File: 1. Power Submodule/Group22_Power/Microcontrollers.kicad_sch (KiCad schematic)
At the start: 3 parts, among them J4 Conn_01x08_Male, J5 Conn_01x08_Male, J7 GPIO

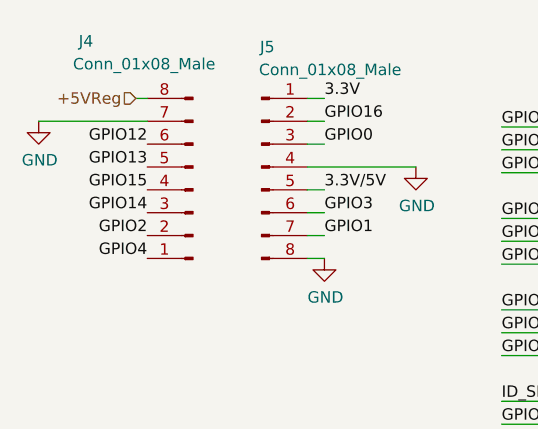
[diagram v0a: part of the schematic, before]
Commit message: $1
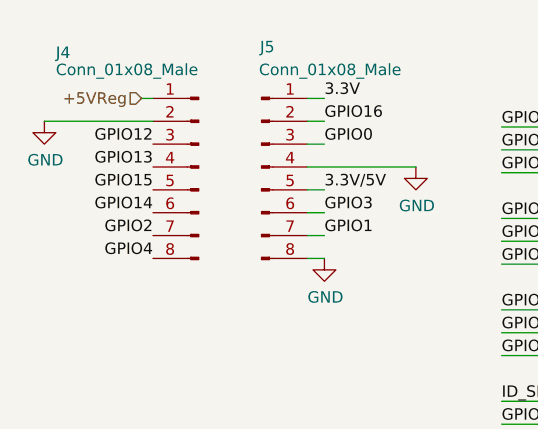
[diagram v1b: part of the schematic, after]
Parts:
- J4, J5: footprint Connector_PinHeader_2.54mm:PinHeader_1x08_P2.54mm_Vertical -> Connector_PinSocket_2.54mm:PinSocket_1x08_P2.54mm_Vertical
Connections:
- net +5VReg: now also J4.1 (Pin_1); no longer J4.8 (Pin_8)
- net GND: now also J4.2 (Pin_2); no longer J4.7 (Pin_7)
- net GPIO12: now also J4.3 (Pin_3); no longer J4.6 (Pin_6)
- net GPIO13: now also J4.4 (Pin_4); no longer J4.5 (Pin_5)
- net GPIO14: now also J4.6 (Pin_6); no longer J4.3 (Pin_3)
- net GPIO15: now also J4.5 (Pin_5); no longer J4.4 (Pin_4)
- net GPIO2: now also J4.7 (Pin_7); no longer J4.2 (Pin_2)
- net GPIO4: now also J4.8 (Pin_8); no longer J4.1 (Pin_1)
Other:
- moved on the sheet: J4
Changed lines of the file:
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@@
     (stroke (width 0) (type solid) (color 0 0 0 0))
-  )
-  (wire (pts (xy 166.37 97.79) (xy 167.64 97.79))
-    (stroke (width 0) (type default) (color 0 0 0 0))
   )
   (wire (pts (xy 248.92 144.145) (xy 275.59 144.145))
@@
     (stroke (width 0) (type default) (color 0 0 0 0))
   )
+  (wire (pts (xy 156.21 100.33) (xy 168.275 100.33))
+    (stroke (width 0) (type default) (color 0 0 0 0))
+  )
   (wire (pts (xy 251.46 90.17) (xy 251.46 98.425))
     (stroke (width 0) (type solid) (color 0 0 0 0))
@@
     (stroke (width 0) (type solid) (color 0 0 0 0))
   )
+  (wire (pts (xy 167.005 97.79) (xy 168.275 97.79))
+    (stroke (width 0) (type default) (color 0 0 0 0))
+  )
   (wire (pts (xy 236.22 121.285) (xy 207.01 121.285))
     (stroke (width 0) (type solid) (color 0 0 0 0))
@@
     (stroke (width 0) (type solid) (color 0 0 0 0))
   )
-  (wire (pts (xy 155.575 100.33) (xy 167.64 100.33))
-    (stroke (width 0) (type default) (color 0 0 0 0))
-  )
   (wire (pts (xy 231.14 98.425) (xy 236.22 98.425))
     (stroke (width 0) (type solid) (color 0 0 0 0))
@@
     (effects (font (size 1.27 1.27)) (justify left bottom))
   )
-  (label "GPIO4" (at 167.64 115.57 180)
-    (effects (font (size 1.27 1.27)) (justify right bottom))
-  )
-  (label "GPIO12" (at 167.64 102.87 180)
+  (label "GPIO13" (at 168.275 105.41 180)
     (effects (font (size 1.27 1.27)) (justify right bottom))
   )
@@
     (effects (font (size 1.27 1.27)) (justify left bottom))
   )
-  (label "GPIO13" (at 167.64 105.41 180)
-    (effects (font (size 1.27 1.27)) (justify right bottom))
-  )
   (label "GPIO0" (at 187.325 102.87 0)
     (effects (font (size 1.27 1.27)) (justify left bottom))
   )
+  (label "GPIO12" (at 168.275 102.87 180)
+    (effects (font (size 1.27 1.27)) (justify right bottom))
+  )
   (label "GPIO1" (at 187.325 113.03 0)
     (effects (font (size 1.27 1.27)) (justify left bottom))
@@
     (effects (font (size 1.27 1.27)) (justify left bottom))
   )
+  (label "GPIO2" (at 168.275 113.03 180)
+    (effects (font (size 1.27 1.27)) (justify right bottom))
+  )
   (label "GPIO[24]" (at 275.59 118.745 180)
     (effects (font (size 1.27 1.27)) (justify right bottom))
@@
     (effects (font (size 1.27 1.27)) (justify right bottom))
   )
-  (label "GPIO15" (at 167.64 107.95 180)
+  (label "GPIO14" (at 168.275 110.49 180)
     (effects (font (size 1.27 1.27)) (justify right bottom))
   )
@@
     (effects (font (size 1.27 1.27)) (justify left bottom))
   )
+  (label "GPIO4" (at 168.275 115.57 180)
+    (effects (font (size 1.27 1.27)) (justify right bottom))
+  )
   (label "GPIO[27]" (at 207.01 113.665 0)
     (effects (font (size 1.27 1.27)) (justify left bottom))
@@
     (effects (font (size 1.27 1.27)) (justify left bottom))
   )
-  (label "GPIO2" (at 167.64 113.03 180)
+  (label "GPIO15" (at 168.275 107.95 180)
     (effects (font (size 1.27 1.27)) (justify right bottom))
   )
@@
     (effects (font (size 1.27 1.27)) (justify right bottom))
   )
-  (label "GPIO14" (at 167.64 110.49 180)
-    (effects (font (size 1.27 1.27)) (justify right bottom))
-  )
   (label "GPIO[5]" (at 207.01 133.985 0)
     (effects (font (size 1.27 1.27)) (justify left bottom))
@@
     (effects (font (size 1.27 1.27)) (justify left bottom))
   )
-  (hierarchical_label "+5VReg" (shape input) (at 166.37 97.79 180)
+  (hierarchical_label "+5VReg" (shape input) (at 167.005 97.79 180)
     (effects (font (size 1.27 1.27)) (justify right))
   )
@@
     (property "Reference" "J5" (id 0) (at 180.975 92.075 0))
     (property "Value" "Conn_01x08_Male" (id 1) (at 187.96 94.615 0))
-    (property "Footprint" "Connector_PinHeader_2.54mm:PinHeader_1x08_P2.54mm_Vertical" (id 2) (at 180.34 105.41 0)
+    (property "Footprint" "Connector_PinSocket_2.54mm:PinSocket_1x08_P2.54mm_Vertical" (id 2) (at 180.34 105.41 0)
       (effects (font (size 1.27 1.27)) hide)
     )
@@
     (pin "8")
   )
-  (symbol (lib_id "Connector:Conn_01x08_Male") (at 172.72 107.95 180) (unit 1)
-    (in_bom yes) (on_board yes)
-    (property "Reference" "J4" (id 0) (at 160.02 91.44 0)
+  (symbol (lib_id "Connector:Conn_01x08_Male") (at 173.355 105.41 0) (mirror y) (unit 1)
+    (in_bom yes) (on_board yes)
+    (property "Reference" "J4" (id 0) (at 157.48 92.71 0)
       (effects (font (size 1.27 1.27)) (justify right))
     )
-    (property "Value" "Conn_01x08_Male" (id 1) (at 159.385 93.98 0)
+    (property "Value" "Conn_01x08_Male" (id 1) (at 157.48 94.615 0)
       (effects (font (size 1.27 1.27)) (justify right))
     )
-    (property "Footprint" "Connector_PinHeader_2.54mm:PinHeader_1x08_P2.54mm_Vertical" (id 2) (at 172.72 107.95 0)
-      (effects (font (size 1.27 1.27)) hide)
-    )
-    (property "Datasheet" "~" (id 3) (at 172.72 107.95 0)
+    (property "Footprint" "Connector_PinSocket_2.54mm:PinSocket_1x08_P2.54mm_Vertical" (id 2) (at 173.355 105.41 0)
+      (effects (font (size 1.27 1.27)) hide)
+    )
+    (property "Datasheet" "~" (id 3) (at 173.355 105.41 0)
       (effects (font (size 1.27 1.27)) hide)
     )
@@
     (pin "1")
   )
-  (symbol (lib_id "power:GND") (at 155.575 100.33 0) (unit 1)
-    (in_bom yes) (on_board yes)
-    (property "Reference" "#PWR0103" (id 0) (at 155.575 106.68 0)
-      (effects (font (size 1.27 1.27)) hide)
-    )
-    (property "Value" "GND" (id 1) (at 155.6893 104.6544 0))
-    (property "Footprint" "" (id 2) (at 155.575 100.33 0))
-    (property "Datasheet" "" (id 3) (at 155.575 100.33 0))
-    (pin "1")
-  )
   (symbol (lib_id "power:GND") (at 233.68 150.495 0) (unit 1)
     (in_bom yes) (on_board yes)
@@
     (pin "1")
   )
+  (symbol (lib_id "power:GND") (at 156.21 100.33 0) (unit 1)
+    (in_bom yes) (on_board yes)
+    (property "Reference" "#PWR0103" (id 0) (at 156.21 106.68 0)
+      (effects (font (size 1.27 1.27)) hide)
+    )
+    (property "Value" "GND" (id 1) (at 156.3243 104.6544 0))
+    (property "Footprint" "" (id 2) (at 156.21 100.33 0))
+    (property "Datasheet" "" (id 3) (at 156.21 100.33 0))
+    (pin "1")
+  )

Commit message: $1
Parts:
- J4, J5, J7: Populate (none) -> No
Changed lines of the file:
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@@
+      (effects (font (size 1.27 1.27)) hide)
+    )
+    (property "Populate" "No" (id 4) (at 180.34 105.41 0)
       (effects (font (size 1.27 1.27)) hide)
     )
@@
       (effects (font (size 1.27 1.27)) hide)
     )
+    (property "Populate" "No" (id 4) (at 173.355 105.41 0)
+      (effects (font (size 1.27 1.27)) hide)
+    )
     (pin "1")
     (pin "2")
@@
       (effects (font (size 1.27 1.27)) hide)
     )
+    (property "Populate" "No" (id 4) (at 241.3 121.285 0)
+      (effects (font (size 1.27 1.27)) hide)
+    )
